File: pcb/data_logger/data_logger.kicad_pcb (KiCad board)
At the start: 2 copper layers, 50 x 50 mm, 1 part, among them U1 ESP32-WROOM-32

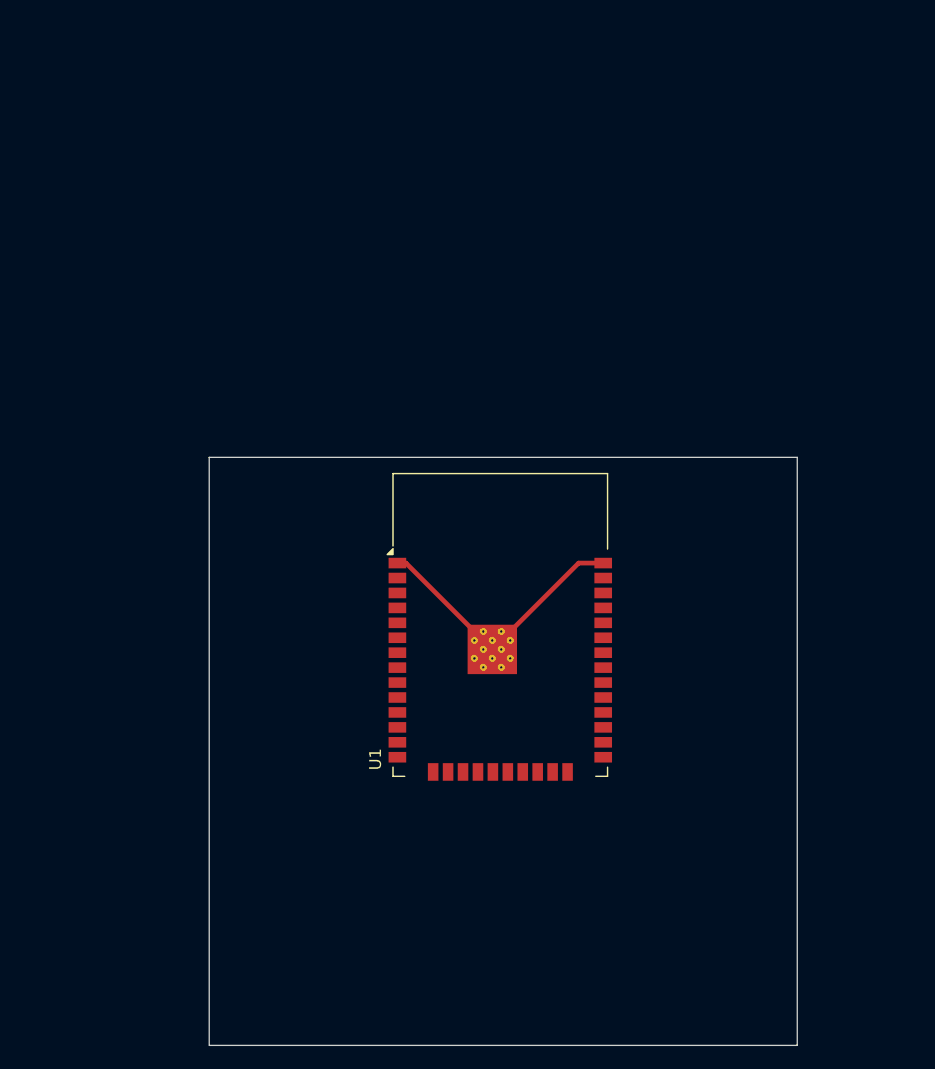
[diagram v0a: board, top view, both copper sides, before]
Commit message: alles sauber
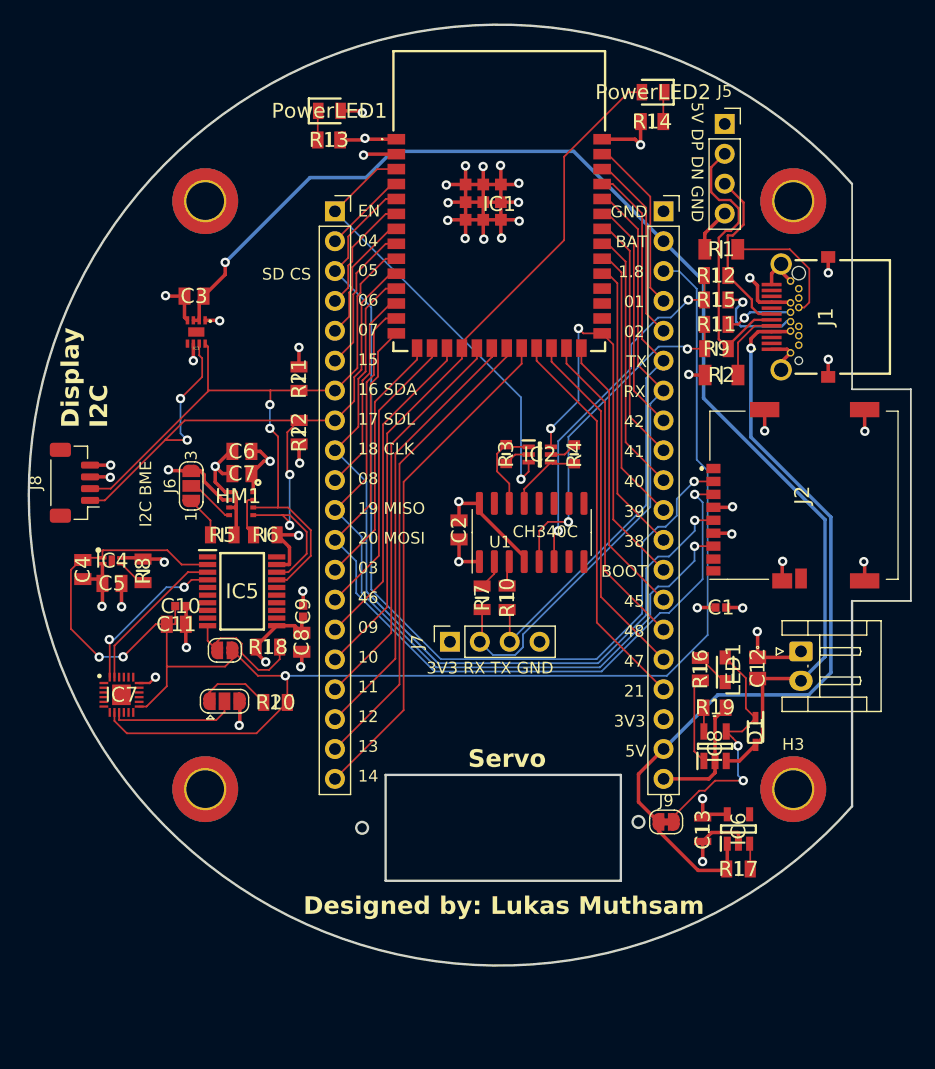
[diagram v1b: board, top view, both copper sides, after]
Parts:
- added C1: 10uF, C10uF:CAPC1005X70N, F.Cu at (82.5, 73.8)
- added C10: C10uF, C10uF:CAPC1005X70N, F.Cu at (36.6, 73.7)
- added C11: 01.uF, C0.1uF:CAPC2012X94N, F.Cu at (36.2, 75.2)
- added C12: C4.7uF, C4.7uF:C0805, F.Cu at (85.6, 78.9)
- added C13: C2.2uF, C2.2uF:CAPC2012X145N, F.Cu at (81.0, 92.7)
- added C2: 08055C104KAT2A, C0.1uF:CAPC2012X94N, F.Cu at (60.2, 67.2)
- added C3: 08055C104KAT2A, C0.1uF:CAPC2012X94N, F.Cu at (37.7, 47.3)
- added C4: 1uF, C1uF:CAPC2012X140N, F.Cu at (28.2, 70.5)
- added C5: 1uF, C1uF:CAPC2012X140N, F.Cu at (30.7, 71.7)
- added C6: 0.1uF, C0.1uF:CAPC2012X94N, F.Cu at (41.8, 60.5)
- added C7: 0.1uF, C0.1uF:CAPC2012X94N, F.Cu at (41.8, 62.4)
- added C8: 01.uF, C0.1uF:CAPC2012X94N, F.Cu at (46.9, 76.7)
- added C9: C10uF, C10uF:CAPC1005X70N, F.Cu at (47.0, 74.1)
- added D1: 3A-10V-280mV, D-3A-10V-300mV:SOD2513X110N, F.Cu at (85.5, 84.3)
- added H1: MountingHole_Pad, MountingHole:MountingHole_3.2mm_M3_DIN965_Pad_TopBottom, F.Cu at (38.7, 39.2)
- added H2: MountingHole_Pad, MountingHole:MountingHole_3.2mm_M3_DIN965_Pad_TopBottom, F.Cu at (38.7, 89.2)
- added H3: MountingHole_Pad, MountingHole:MountingHole_3.2mm_M3_DIN965_Pad_TopBottom, F.Cu at (88.7, 89.2)
- added H4: MountingHole_Pad, MountingHole:MountingHole_3.2mm_M3_DIN965_Pad_TopBottom, F.Cu at (88.7, 39.2)
- added HM1: BME280, BME280:BME280, F.Cu at (40.7, 64.0)
- added IC1: ESP32-S3-WROOM-2-N32R8V, ESP32-S3-WROOM-2:ESP32S3WROOM2N32R8V, F.Cu at (63.7, 39.2)
- added IC2: MBT3904DW1T1G, MBT3904DW1T1G:SOT65P210X110-6N, F.Cu at (67.1, 60.8)
- added IC3: MAX17048G+T10, sparkfun_import:DFN-8, F.Cu at (37.9, 50.3)
- added IC4: MIC94310-GYMT-TR, MIC94310-GYMT-TR:SON50P155X120X60-5N-D, F.Cu at (30.7, 69.8)
- added IC5: TXS0108EQPWRQ1, TXS0108E:SOP65P640X120-20N, F.Cu at (41.8, 72.4)
- added IC6: AP2112K-3.3TRG1, AP2112K-3.3V:SOT95P282X130-5N, F.Cu at (84.0, 92.6)
- added IC7: ICM-20948, ICM-20948:QFN40P300X300X105-25N-D, F.Cu at (31.5, 81.2)
- added IC8: MCP73831T-2ACI_OT, MCP73831:SOT95P270X145-5N, F.Cu at (82.0, 85.6)
- added J1: UJ32-C-H-G-H2-SMT-TR, USB-C:UJ32CHGH2SMTTR, F.Cu at (91.9, 49.1)
- added J10: TXS0108E, Jumper:SolderJumper-2_P1.3mm_Open_RoundedPad1.0x1.5mm, F.Cu at (40.3, 77.4)
- added J11: 1769, Connector_JST:JST_EH_S2B-EH_1x02_P2.50mm_Horizontal, F.Cu at (89.3, 77.5)
- added J12: ~, Jumper:SolderJumper-3_P1.3mm_Open_RoundedPad1.0x1.5mm, F.Cu at (40.3, 81.7)
- added J2: 045138008100858+, SD-Card-Slot-2:045138008100858, F.Cu at (89.4, 64.2)
- added J3: Conn_01x20_Pin, Connector_PinSocket_2.54mm:PinSocket_1x20_P2.54mm_Vertical, F.Cu at (49.7, 40.1)
- added J4: Conn_01x20_Pin, Connector_PinSocket_2.54mm:PinSocket_1x20_P2.54mm_Vertical, F.Cu at (77.6, 40.1)
- added J5: Conn_01x04, Connector_PinSocket_2.54mm:PinSocket_1x04_P2.54mm_Vertical, F.Cu at (82.8, 32.6)
- added J6: Conn_01x03_Pin, Jumper:SolderJumper-3_P1.3mm_Open_RoundedPad1.0x1.5mm_NumberLabels, F.Cu at (37.5, 63.4)
- added J7: Conn_01x04, Connector_PinSocket_2.54mm:PinSocket_1x04_P2.54mm_Vertical, F.Cu at (59.5, 76.7)
- added J8: Conn_01x04, Connector_JST:JST_SH_BM04B-SRSS-TB_1x04-1MP_P1.00mm_Vertical, F.Cu at (27.5, 63.2)
- added J9: LiPo, Jumper:SolderJumper-2_P1.3mm_Bridged_RoundedPad1.0x1.5mm, F.Cu at (77.8, 92.0)
- added LED1: VLMY234ABCA-GS08, LED-yellow:LEDM2214X140N, F.Cu at (82.9, 79.1)
- added PowerLED1: 150080RS75000, LED-red:LEDC2012X80N, F.Cu at (49.2, 31.5)
- added PowerLED2: 150080RS75000, LED-red:LEDC2012X80N, F.Cu at (76.7, 29.9)
- added R1: 5.1k, R5.1k:RESC3116X65N, F.Cu at (82.5, 43.3)
- added R10: R0, R0:RESC2013X84N, F.Cu at (64.3, 72.9)
- added R11: R0, R0:RESC2013X84N, F.Cu at (82.1, 49.7)
- added R12: R0, R0:RESC2013X84N, F.Cu at (82.1, 45.5)
- added R13: MCU0805MD1000BP100, R1k:RESC2012X55N, F.Cu at (49.2, 34.0)
- added R14: MCU0805MD1000BP100, R1k:RESC2012X55N, F.Cu at (76.7, 32.5)
- added R15: R0, R0:RESC2013X84N, F.Cu at (82.1, 47.6)
- added R16: MCU0805MD1000BP100, R1k:RESC2012X55N, F.Cu at (80.8, 79.0)
- added R17: 330k, R330k:RESC2012X50N, F.Cu at (84.0, 96.0)
- added R18: 330k, R330k:RESC2012X50N, F.Cu at (44.0, 77.1)
- added R19: R2.2k, R2.2k:RESC2013X65N, F.Cu at (82.0, 82.3)
- added R2: 5.1k, R5.1k:RESC3116X65N, F.Cu at (82.6, 54.0)
- added R20: R4.7k, R4.7k:RESC2012X50N, F.Cu at (44.6, 81.8)
- added R21: R4.7k, R4.7k:RESC2012X50N, F.Cu at (46.6, 54.3)
- added R22: R4.7k, R4.7k:RESC2012X50N, F.Cu at (46.6, 58.9)
- added R3: 10k, R10k:RESC1608X55N, F.Cu at (64.2, 60.7)
- added R4: 10k, R10k:RESC1608X55N, F.Cu at (70.0, 60.7)
- added R5: R4.7k, R4.7k:RESC2012X50N, F.Cu at (40.1, 67.6)
- added R6: R4.7k, R4.7k:RESC2012X50N, F.Cu at (43.8, 67.6)
- added R7: R0, R0:RESC2013X84N, F.Cu at (62.2, 72.9)
- added R8: R4.7k, R4.7k:RESC2012X50N, F.Cu at (33.4, 70.7)
- added R9: R0, R0:RESC2013X84N, F.Cu at (82.1, 51.8)
- U1: value ESP32-WROOM-32 -> CH340C; footprint RF_Module:ESP32-WROOM-32 -> Package_SO:SOIC-16_3.9x9.9mm_P1.27mm
- moved U1 11.2 mm to (66.4, 67.4), turned to 90 degrees
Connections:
- U1 pad 13: unconnected-(U1-IO14-Pad13) -> /CH340_DTR
- U1 pad 14: unconnected-(U1-IO12-Pad14) -> /CH340_RTS
- U1 pad 15: GND -> unconnected-(U1-R232-Pad15)
- U1 pad 16: unconnected-(U1-IO13-Pad16) -> +3V3
- U1 pad 2: +3V3 -> Net-(U1-TXD)
- U1 pad 3: unconnected-(U1-EN-Pad3) -> Net-(U1-RXD)
- U1 pad 4: unconnected-(U1-SENSOR_VP-Pad4) -> +3V3
- U1 pad 5: unconnected-(U1-SENSOR_VN-Pad5) -> Net-(U1-UD+)
- U1 pad 6: unconnected-(U1-IO34-Pad6) -> Net-(U1-UD-)
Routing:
- net +1V8: track 0.00 -> 140.9 mm, vias 0 -> 3
- net GND: track 19.3 -> 143.2 mm, vias 0 -> 37
- net +3V8: track 0.00 -> 107.5 mm, vias 0 -> 1
- net /GPIO5_CS: track 0.00 -> 79.3 mm, vias 0 -> 1
- net +5V: track 0.00 -> 74.8 mm, vias 0 -> 2
- net /SCL: track 0.00 -> 70.5 mm, vias 0 -> 4
- net /GPIO20_MOSI: track 0.00 -> 69.5 mm, vias 0 -> 1
- net /GPIO18_CLK: track 0.00 -> 69.5 mm, vias 0 -> 1
- net /GPIO19_MISO: track 0.00 -> 65.6 mm, vias 0 -> 1
- net /SDA: track 0.00 -> 64.2 mm, vias 0 -> 2
- net /GPIO10: track 0.00 -> 59.7 mm
- net +3V3: track 0.00 -> 52.8 mm, vias 0 -> 15
- net /CHIP_RX: track 0.00 -> 52.7 mm
- net /CHIP_TX: track 0.00 -> 50.2 mm
- net /GPIO14: track 0.00 -> 43.2 mm
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- added copper zone on In1.Cu, net +3V3
- added copper zone on In1.Cu, net +5V
- added copper zone on In2.Cu, net GND
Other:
- board size 50 x 50 mm -> 75 x 80 mm
- copper layers 2 -> 4
- board text added: "+"
- board text added: "-"
- board text added: "01"
- board text added: "02"
- board text added: "03"
- board text added: "04"
- board text added: "05"
- board text added: "06"
- board text added: "07"
- board text added: "08"
- board text added: "09"
- board text added: "1.8"
- board text added: "10"
- board text added: "11"
- board text added: "12"
- board text added: "13"
- board text added: "14"
- board text added: "15"
- board text added: "16 SDA"
- board text added: "17 SDL"
- board text added: "18 CLK"
- board text added: "19 MISO"
- board text added: "20 MOSI"
- board text added: "21"
- board text added: "38"
- board text added: "39"
- board text added: "3V3"
- board text added: "3V3 RX TX GND"
- board text added: "40"
- board text added: "41"
- board text added: "42"
- board text added: "45"
- board text added: "46"
- board text added: "47"
- board text added: "48"
- board text added: "5V"
- board text added: "5V DP DN GND"
- board text added: "BAT"
- board text added: "BOOT"
- board text added: "CH340C"
- board text added: "Designed by: Lukas Muthsam"
- board text added: "Display I2C"
- board text added: "EN"
- board text added: "GND"
- board text added: "I2C BME"
- board text added: "RX"
- board text added: "SD CS"
- board text added: "Servo"
- board text added: "TX"
